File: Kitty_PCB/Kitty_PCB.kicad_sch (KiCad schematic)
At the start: 30 parts, among them J1 Vin, J10 GND, J11 GND, J12 GND, J13 3v3, J14 GND, J15 GND, J2 HC-05, J3 10V, J4 Batt, J5 GND, J6 Vin, J7 10V, J8 GPIOs, J9 Bluefruit_LE, SW1 Vin_Switch, U1 PicoW, U2 Voltage Regulator

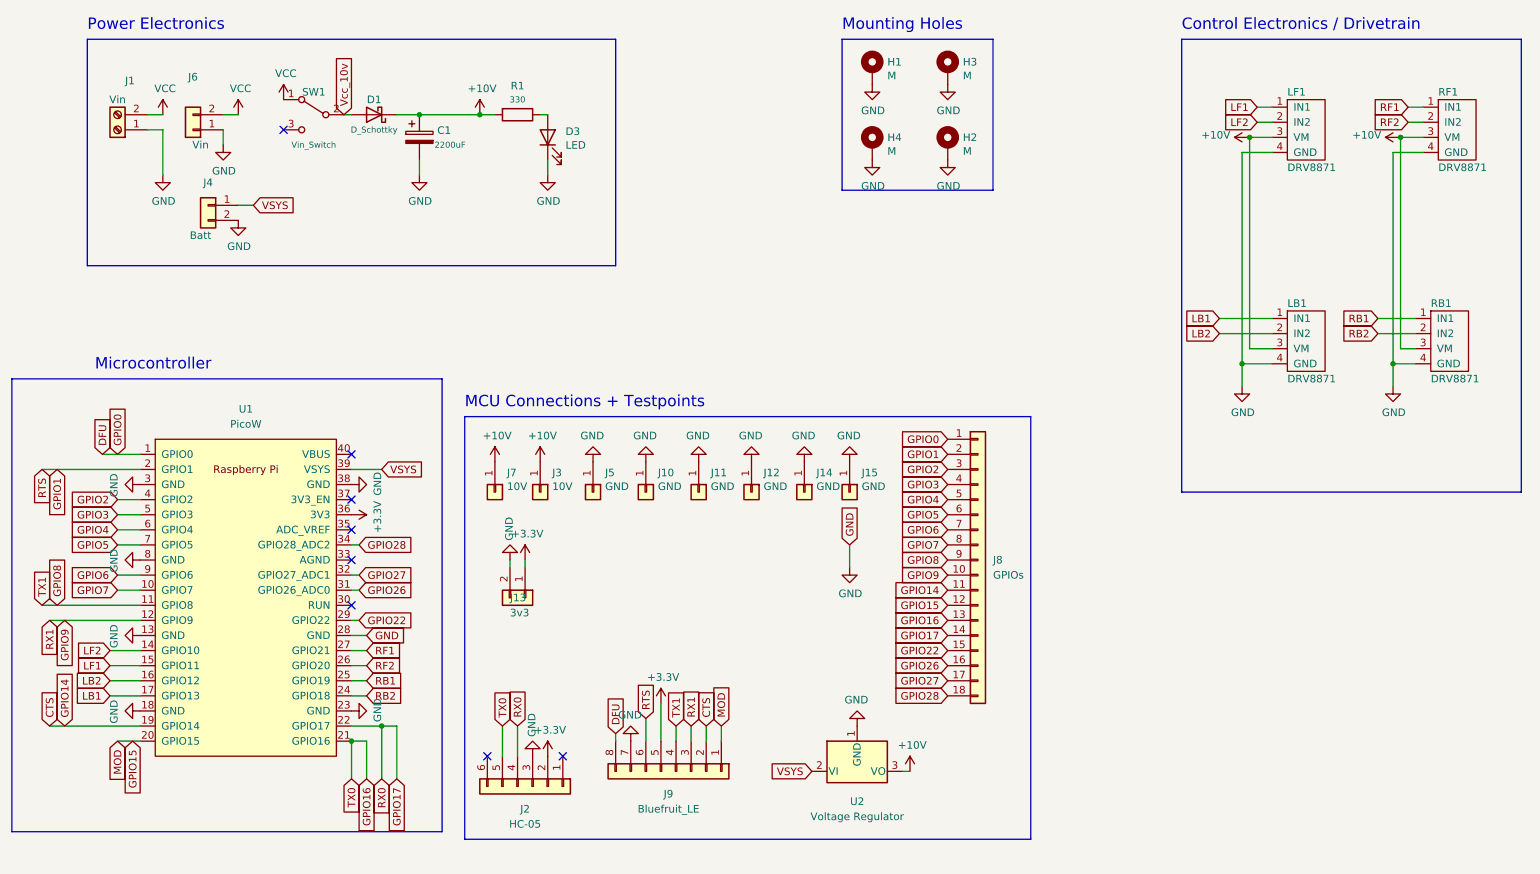
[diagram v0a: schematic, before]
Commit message: Edits
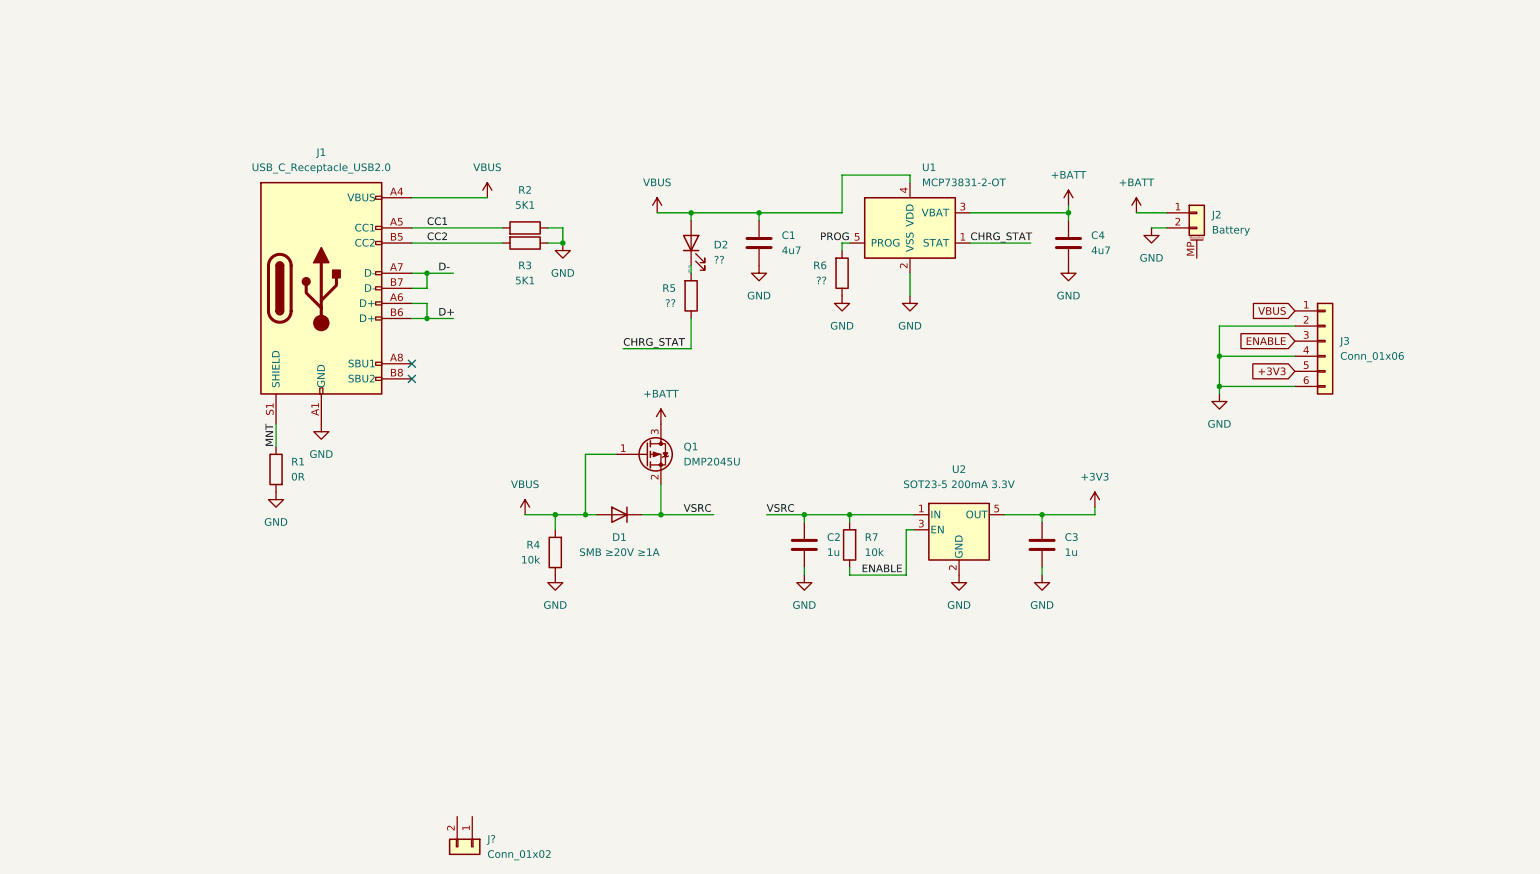
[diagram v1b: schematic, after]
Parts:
- removed C1: 2200uF, Capacitor_THT:CP_Radial_D10.0mm_P5.00mm, symbol M5_BuggyProject-rescue:CP-Device
- removed D1: D_Schottky, Package_TO_SOT_THT:TO-220-2_Vertical, symbol Device:D_Schottky
- removed D3: LED, LED_THT:LED_D3.0mm, symbol Device:LED
- removed H1, H2, H3, H4: M, MountingHole:MountingHole_4.3mm_M4_Pad_Via, symbol Mechanical:MountingHole_Pad
- removed J1: Vin, Connector_AMASS:AMASS_XT60-M_1x02_P7.20mm_Vertical, symbol Connector:Screw_Terminal_01x02
- removed J10, J11, J12, J14, J15, J5: GND, TestPoint:TestPoint_Plated_Hole_D5.0mm, symbol Connector_Generic:Conn_01x01
- removed J13: 3v3, Connector_PinSocket_2.54mm:PinSocket_1x02_P2.54mm_Vertical, symbol Connector_Generic:Conn_01x02
- removed J2: HC-05, Connector_PinSocket_2.54mm:PinSocket_1x06_P2.54mm_Vertical, symbol Connector_Generic:Conn_01x06
- removed J3, J7: 10V, TestPoint:TestPoint_Plated_Hole_D5.0mm, symbol Connector_Generic:Conn_01x01
- removed J4: Batt, Connector_PinSocket_2.54mm:PinSocket_1x02_P2.54mm_Vertical, symbol Connector_Generic:Conn_01x02
- removed J6: Vin, Connector_PinSocket_2.54mm:PinSocket_1x02_P2.54mm_Vertical, symbol Connector_Generic:Conn_01x02
- removed J8: GPIOs, Connector_PinSocket_2.54mm:PinSocket_1x18_P2.54mm_Vertical, symbol Connector_Generic:Conn_01x18
- removed J9: Bluefruit_LE, Connector_PinSocket_2.54mm:PinSocket_1x08_P2.54mm_Vertical, symbol Connector_Generic:Conn_01x08
- removed LB1, LF1, RB1, RF1: DRV8871, Connector_PinSocket_2.54mm:PinSocket_1x04_P2.54mm_Vertical, symbol Buggy_Components:Adafruit_DRV8871_Breakout
- removed SW1: Vin_Switch, Buggy_Footprints:1101M2S3CQE2, symbol Switch:SW_SPDT
- removed U1: PicoW, RPi_Pico:RPi_PicoW_SMD_TH, symbol RPi_Pico:PicoW
- removed U2: Voltage Regulator, Package_TO_SOT_THT:TO-220-3_Vertical, symbol Regulator_Linear:MC79M15_TO220
- added C1, C4: 4u7, Capacitor_SMD:C_0805_2012Metric_Pad1.18x1.45mm_HandSolder, symbol Device:C
- added C2, C3: 1u, Capacitor_SMD:C_0805_2012Metric_Pad1.18x1.45mm_HandSolder, symbol Device:C
- added D1: SMB ≥20V ≥1A, Diode_SMD:D_1206_3216Metric_Pad1.42x1.75mm_HandSolder, symbol Device:D
- added D2: ??, LED_SMD:LED_0805_2012Metric_Pad1.15x1.40mm_HandSolder, symbol Device:LED
- added J1: USB_C_Receptacle_USB2.0, Connector_USB:USB_C_Receptacle_Palconn_UTC16-G, symbol Connector:USB_C_Receptacle_USB2.0
- added J2: Battery, Connector_JST:JST_PH_S2B-PH-SM4-TB_1x02-1MP_P2.00mm_Horizontal, symbol Connector_Generic_MountingPin:Conn_01x02_MountingPin
- added J3: Conn_01x06, Connector_PinHeader_2.54mm:PinHeader_1x06_P2.54mm_Vertical, symbol Connector_Generic:Conn_01x06
- added J?: Conn_01x02, symbol Connector_Generic:Conn_01x02
- added Q1: DMP2045U, Package_TO_SOT_SMD:SOT-23, symbol Transistor_FET:AO3401A
- added R2, R3: 5K1, Resistor_SMD:R_0805_2012Metric_Pad1.20x1.40mm_HandSolder, symbol Device:R
- added R4, R7: 10k, Resistor_SMD:R_0805_2012Metric_Pad1.20x1.40mm_HandSolder, symbol Device:R
- added R5, R6: ??, Resistor_SMD:R_0805_2012Metric_Pad1.20x1.40mm_HandSolder, symbol Device:R
- added U1: MCP73831-2-OT, Package_TO_SOT_SMD:SOT-23-5, symbol Battery_Management:MCP73831-2-OT
- added U2: SOT23-5 200mA 3.3V, Package_TO_SOT_SMD:SOT-23-5, symbol Regulator_Linear:TLV70033_SOT23-5
- R1: value 330 -> 0R; footprint Resistor_THT:R_Axial_DIN0204_L3.6mm_D1.6mm_P7.62mm_Horizontal -> Resistor_SMD:R_0805_2012Metric_Pad1.20x1.40mm_HandSolder
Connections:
- net +10V is gone; now on net GND: R1.2
- net +3V3: now also C3.2, J3.5 (Pin_5), U2.5 (OUT)
- net GND: now also C1.1, C2.2, C3.1, C4.2, J1.A1 (GND), J1.A12 (GND), J1.B1 (GND), J1.B12 (GND), J2.2 (Pin_2), J3.2 (Pin_2), J3.4 (Pin_4), J3.6 (Pin_6), R2.1, R3.1, R4.1, R6.1, U1.2 (VSS), U2.2 (GND)
- net MNT: now reaches R1.1
- net MNT: now also J1.S1 (SHIELD)
- new net +BATT: C4.1, J2.1 (Pin_1), Q1.3 (D), U1.3 (VBAT)
- new net CC1: J1.A5 (CC1), R2.2
- new net CC2: J1.B5 (CC2), R3.2
- new net CHRG_STAT: R5.1, U1.1 (STAT)
- new net D+: J1.A6 (D+), J1.B6 (D+)
- new net D-: J1.A7 (D-), J1.B7 (D-)
- new net ENABLE: J3.3 (Pin_3), R7.1, U2.3 (EN)
- new net LED_D2: D2.1 (K), R5.2
- new net PROG: R6.2, U1.5 (PROG)
- new net VBUS: C1.2, D1.2 (A), D2.2 (A), J1.A4 (VBUS), J1.A9 (VBUS), J1.B4 (VBUS), J1.B9 (VBUS), J3.1 (Pin_1), Q1.1 (G), R4.2, U1.4 (VDD)
- new net VSRC: C2.1, D1.1 (K), Q1.2 (S), R7.2, U2.1 (IN)
- no-connect marks 8 -> 2
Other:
- note removed: "Control Electronics / Drivetrain"
- note removed: "MCU Connections + Testpoints"
- note removed: "Microcontroller"
- note removed: "Mounting Holes"
- note removed: "Power Electronics"
